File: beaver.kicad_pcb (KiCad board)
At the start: 8 copper layers, 31.2 x 44.5 mm, 57 parts, among them J1 Conn_01x04_Male, J2 USB_C_Receptacle_USB2.0, J3 NFC, J4 Conn_01x17, J5 Conn_01x17, SW1 RESET, SW2 USER P0.17, U1 nRF52840, U2 USBLC6-2SC6, U4 AZ1117-3.3, Y1 Crystal_GND24_Small, Y2 Crystal_Small

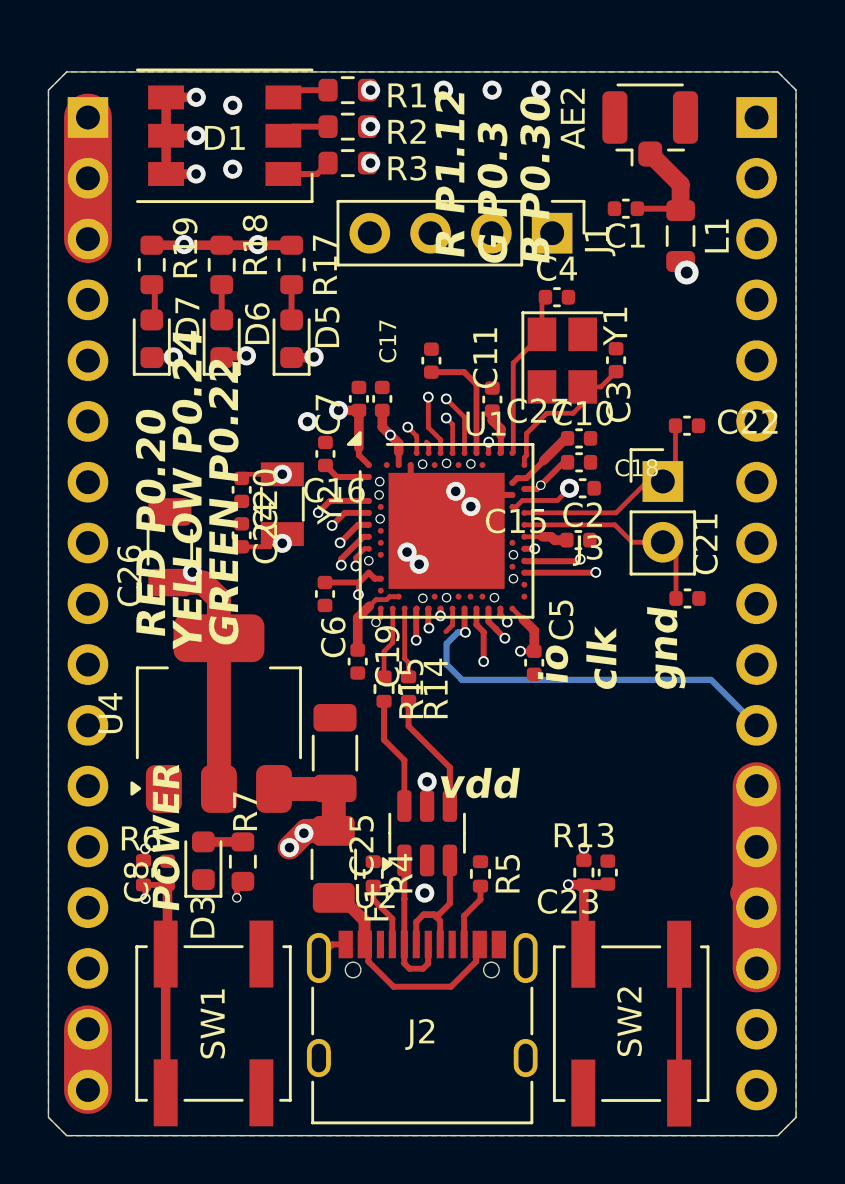
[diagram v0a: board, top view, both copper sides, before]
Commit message: final touches
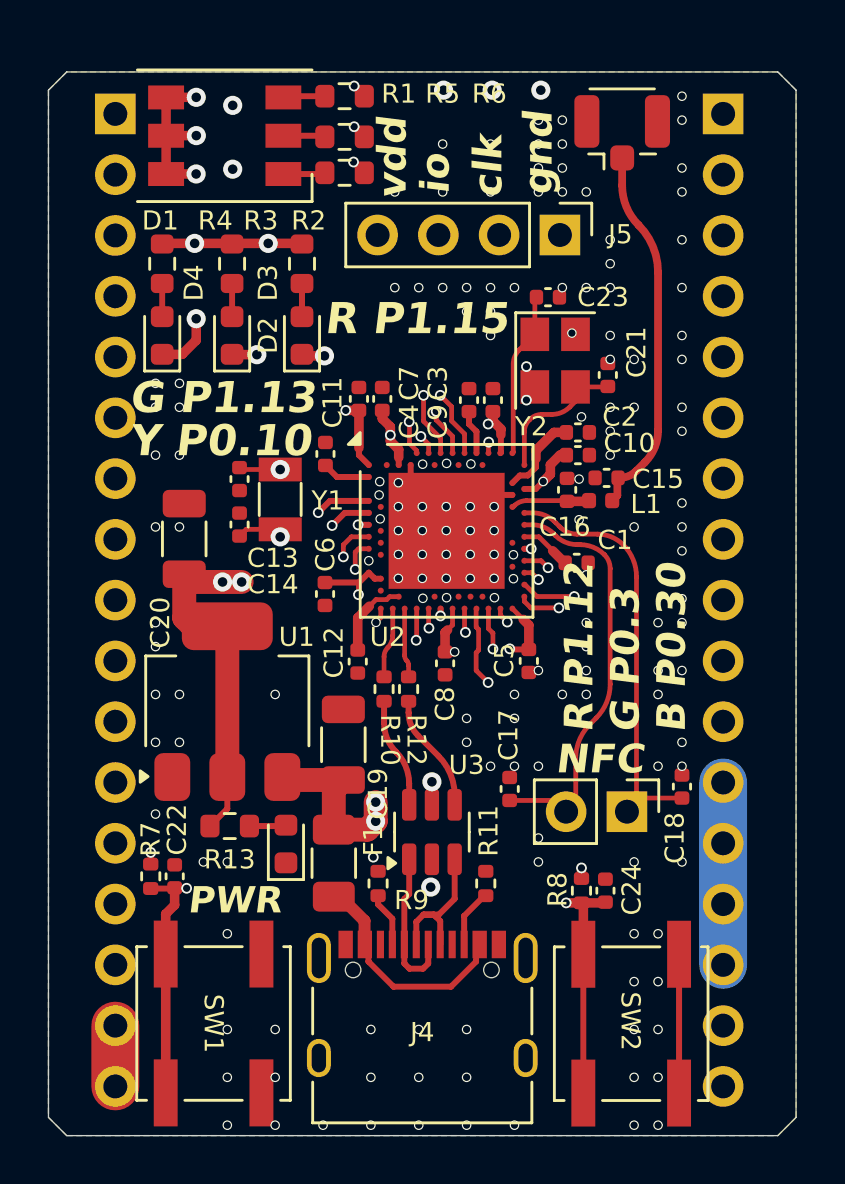
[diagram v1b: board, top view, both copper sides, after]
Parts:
- added C8: 100n, Capacitor_SMD:C_0402_1005Metric, F.Cu at (162.9, 99.0)
- C5, C6, C7: value 1uF -> 100n
- D2: renamed from D5; value YELLOW P0.24 -> Y P0.10
- D3: renamed from D6; value GREEN P0.22 -> G P1.13
- D4: renamed from D7; value RED P0.20 -> R P1.15
- D5: renamed from D3; value POWER -> PWR
- L1: footprint Inductor_SMD:L_0805_2012Metric -> Inductor_SMD:L_0402_1005Metric
- moved C18 15.1 mm to (172.8, 104.2), turned to 90 degrees
- moved J3 13.9 mm to (170.5, 105.2), turned to -90 degrees
- moved L1 11.6 mm to (169.4, 92.2), turned to 180 degrees
- moved C15 11.3 mm to (169.7, 91.3)
- moved C17 10.9 mm to (165.6, 104.3), turned to -90 degrees
- moved D5 3.52 mm to (156.3, 106.6)
- moved C4 2.28 mm to (163.9, 88.0)
- moved R13 1.59 mm to (153.9, 105.8), turned to 180 degrees
- moved J2 1.41 mm to (174.6, 76.1)
- moved AE1 1.18 mm to (170.3, 76.9)
- moved J1 1.15 mm to (149.2, 76.1)
- moved C1 0.95 mm to (168.4, 94.8)
- moved C24 0.76 mm to (169.6, 108.5)
- moved R8 0.76 mm to (168.6, 108.5)
- moved C21 0.71 mm to (169.7, 87.0)
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- renumbered AE2 to AE1, C15 to C1, C18 to C10, C16 to C11, C19 to C12, C20 to C13, C24 to C14, C1 to C15, C2 to C16, C21 to C17, C22 to C18, C25 to C19, C10 to C2, C26 to C20, C3 to C21, C8 to C22, C4 to C23, C23 to C24, C17 to C3, C11 to C4, C27 to C9, J4 to J1, J5 to J2, J2 to J4, J1 to J5, R15 to R10, R5 to R11, R14 to R12, R7 to R13, R17 to R2, R18 to R3, R19 to R4, R2 to R5, R3 to R6, R6 to R7, R13 to R8, R4 to R9, U4 to U1, U1 to U2, U2 to U3, Y2 to Y1, Y1 to Y2
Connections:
- net Net-(AE2-A) renamed /ANT_MATCHED
- net Net-(J1-Pin_2) renamed /SWDCLK
- net Net-(J1-Pin_3) renamed /SWDIO
- net Net-(U1-ANT) renamed /ANT
- Y2 pad 2: unconnected-(Y1-Pad2) -> GNDREF
- Y2 pad 4: unconnected-(Y1-Pad4) -> GNDREF
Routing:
- net /P0.29: track 0.50 -> 26.6 mm, vias 0 -> 1
- net /SWDCLK: track 0.00 -> 20.5 mm, vias 0 -> 1
- net /SWDIO: track 0.00 -> 20.1 mm, vias 0 -> 1
- net /ANT_MATCHED: track 4.36 -> 15.6 mm
- net /ANT: track 13.8 -> 3.30 mm, vias 2 -> 0
- net /NFC-: track 8.88 -> 18.5 mm
- net VDD: track 58.7 -> 49.4 mm, vias 13 -> 14
- net /NFC+: track 8.67 -> 17.6 mm
- net GNDREF: track 20.6 -> 12.5 mm, vias 11 -> 156
- net /USER_BUT: track 18.3 -> 24.6 mm
- net Net-(U2-DEC2): track 4.96 -> 1.86 mm
- net /P1.12: track 25.2 -> 23.2 mm
- net /P0.26: track 12.5 -> 14.1 mm
- net /P0.31: track 17.4 -> 15.9 mm
- net /P0.25: track 14.4 -> 15.9 mm
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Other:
- board text added: "NFC"
- board text added: "R P1.12 G P0.3 B P0.30"
- board text removed: "B P0.30"
- board text removed: "G P0.3"
- board text removed: "R P1.12"
